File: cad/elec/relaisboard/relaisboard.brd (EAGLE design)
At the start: 34 x 23 mm, 28 parts, among them IC1 REG1117, T1 MMUN2233

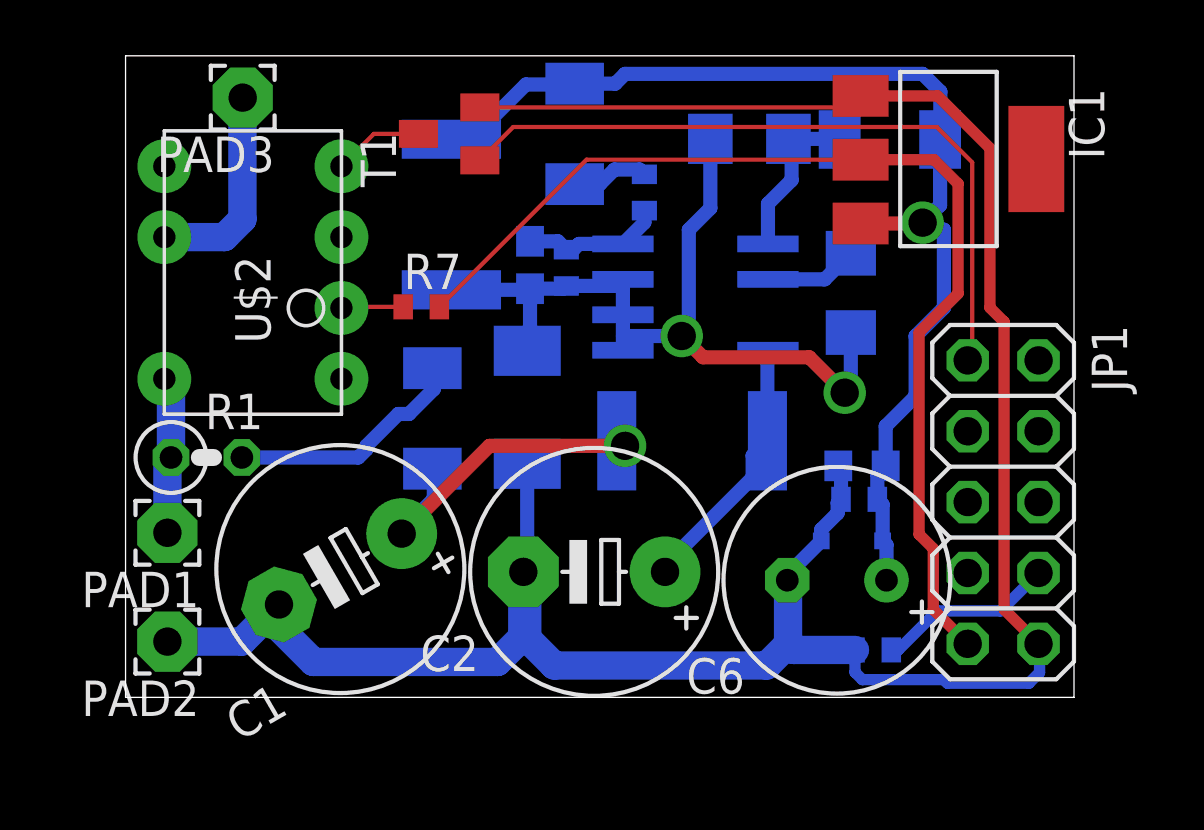
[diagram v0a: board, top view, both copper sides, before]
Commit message: increased cleareance here and there
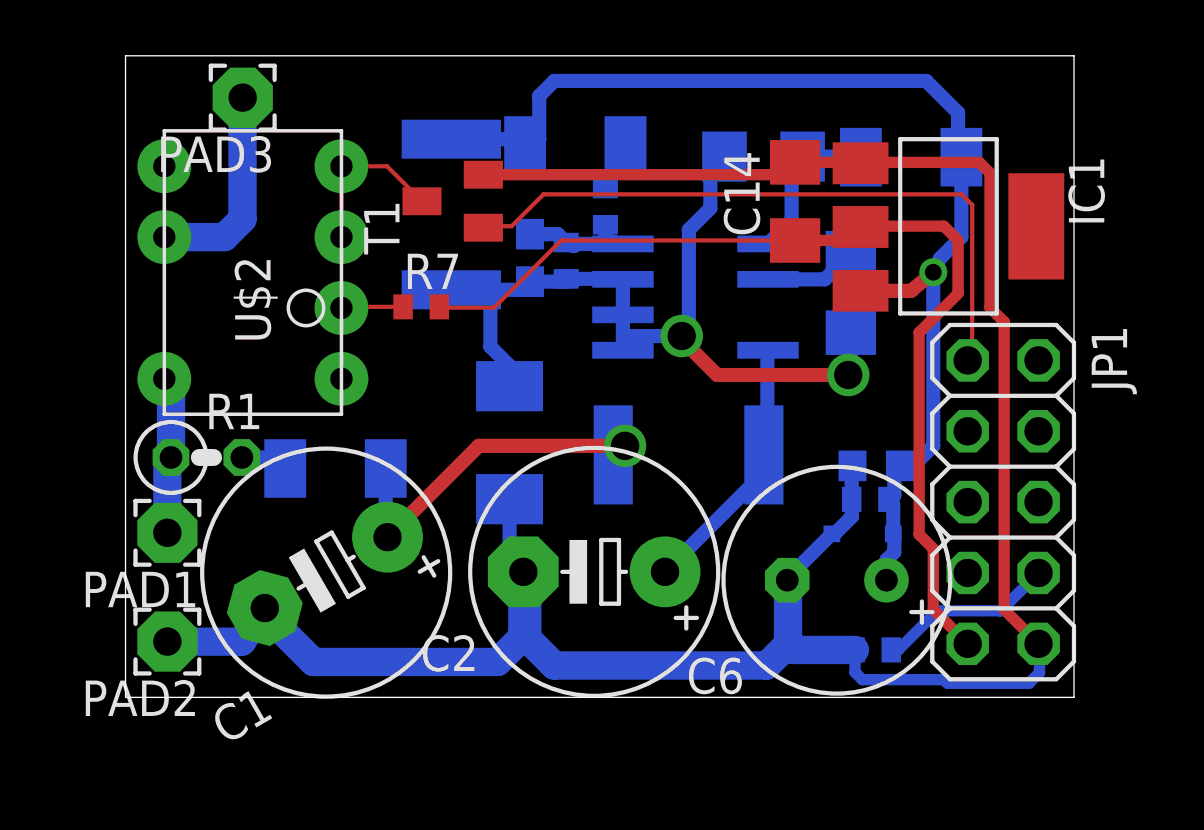
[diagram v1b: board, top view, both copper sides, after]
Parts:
- added C14: 2.2u, rcl:C1206
- moved D1 3.91 mm to (7.53, 8.21), turned to 0 degrees
- moved T1 2.42 mm to (11.7, 17.8)
- moved IC1 2.41 mm to (29.5, 16.9)
- moved R3 1.49 mm to (17.2, 17.6)
- moved D5 1.42 mm to (13.8, 9.13)
- moved D6 0.99 mm to (28.2, 19.4)
- moved C45 0.81 mm to (22.9, 19.4)
- moved C1 0.52 mm to (7.19, 4.47)
- moved L1 0.52 mm to (20.2, 8.69)
- moved R5 0.51 mm to (26.9, 8.30)
- moved DZ7 0.46 mm to (26.4, 5.86)
- moved D4 0.42 mm to (16.1, 19.8), turned to 0 degrees
- moved C7 0.38 mm to (26.7, 7.10)
- moved C3 0.25 mm to (14.5, 15.8)
- moved R2 0.25 mm to (15.8, 15.7)
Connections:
- net +3V3: now also C14.1
- net NEUTRAL: now also C14.2
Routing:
- net N$1: track 8.74 -> 1.76 mm
- net +3V3: track 39.1 -> 36.0 mm
- net N$6: track 3.24 -> 5.95 mm
- net NEUTRAL: track 90.4 -> 87.7 mm
- net IO_0: track 25.8 -> 23.8 mm
- net N$9: track 29.6 -> 30.7 mm
- net N$10: track 2.79 -> 1.94 mm
- net +12V: track 41.6 -> 42.3 mm
- net N$2: track 12.5 -> 13.2 mm
